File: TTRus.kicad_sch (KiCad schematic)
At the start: 90 parts, among them J1 Conn_01x05_Pin, J10 Conn_02x02_Odd_Even, J11 Conn_02x02_Odd_Even, J12 Conn_02x02_Odd_Even, J13 Conn_02x02_Odd_Even, J14 Conn_02x02_Odd_Even, J15 Conn_02x02_Odd_Even, J16 Conn_02x02_Odd_Even, J2 Conn_01x03_Pin, J3 Conn_02x02_Odd_Even, J4 Conn_02x02_Odd_Even, J5 Conn_02x02_Odd_Even, J6 Conn_02x02_Odd_Even, J7 Conn_02x02_Odd_Even, J8 Conn_02x02_Odd_Even, J9 Conn_02x02_Odd_Even, M1 Module:uaefi/0.2, P1 RT-01T-1.0B, P10 RT-01T-1.0B, P11 RT-01T-1.0B, P12 RT-01T-1.0B, P13 RT-01T-1.0B, P14 RT-01T-1.0B, P15 RT-01T-1.0B, P16 RT-01T-1.0B, P17 RT-01T-1.0B, P18 RT-01T-1.0B, P19 RT-01T-1.0B, P2 RT-01T-1.0B, P20 RT-01T-1.0B, P21 RT-01T-1.0B, P22 RT-01T-1.0B, P23 RT-01T-1.0B, P24 RT-01T-1.0B, P25 RT-01T-1.0B, P26 RT-01T-1.0B, P27 RT-01T-1.0B, P28 RT-01T-1.0B, P29 RT-01T-1.0B, P3 RT-01T-1.0B, P30 RT-01T-1.0B, P31 RT-01T-1.0B, P32 RT-01T-1.0B, P33 RT-01T-1.0B, P34 RT-01T-1.0B, P35 RT-01T-1.0B, P36 RT-01T-1.0B, P37 RT-01T-1.0B, P38 RT-01T-1.0B, P39 RT-01T-1.0B, P4 RT-01T-1.0B, P40 RT-01T-1.0B, P41 RT-01T-1.0B, P42 RT-01T-1.0B, P43 RT-01T-1.0B, P44 RT-01T-1.0B, P45 RT-01T-1.0B, P46 RT-01T-1.0B, P47 RT-01T-1.0B, P48 RT-01T-1.0B, P49 RT-01T-1.0B, P5 RT-01T-1.0B, P50 RT-01T-1.0B, P51 RT-01T-1.0B, P52 RT-01T-1.0B, P53 RT-01T-1.0B, P54 RT-01T-1.0B, P55 RT-01T-1.0B, P56 RT-01T-1.0B, P57 RT-01T-1.0B, P58 RT-01T-1.0B, P59 RT-01T-1.0B, P6 RT-01T-1.0B, P60 RT-01T-1.0B, P61 RT-01T-1.0B, P62 RT-01T-1.0B, P63 RT-01T-1.0B, P64 RT-01T-1.0B, P65 RT-01T-1.0B, P66 RT-01T-1.0B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

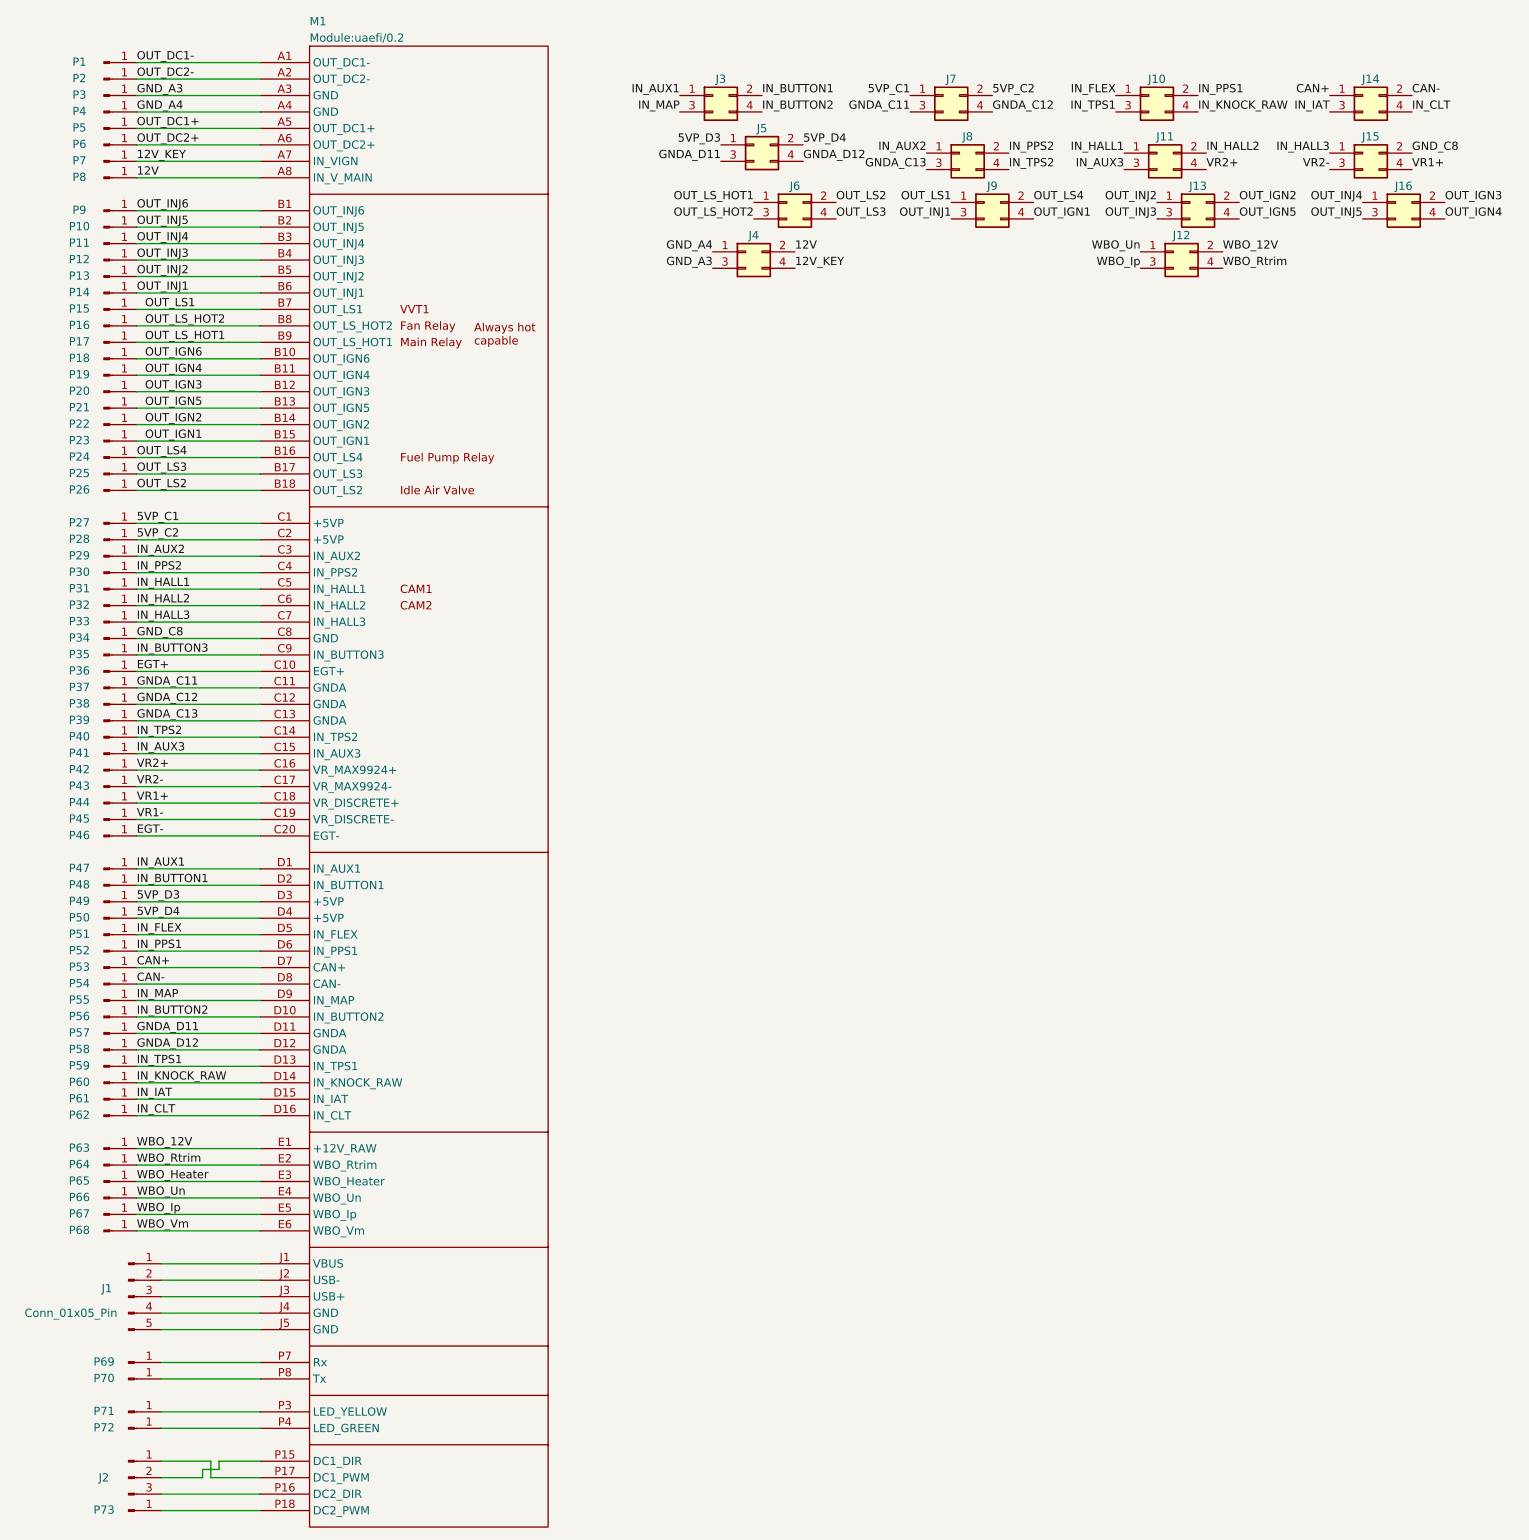
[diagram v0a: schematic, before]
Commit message: Add files via upload
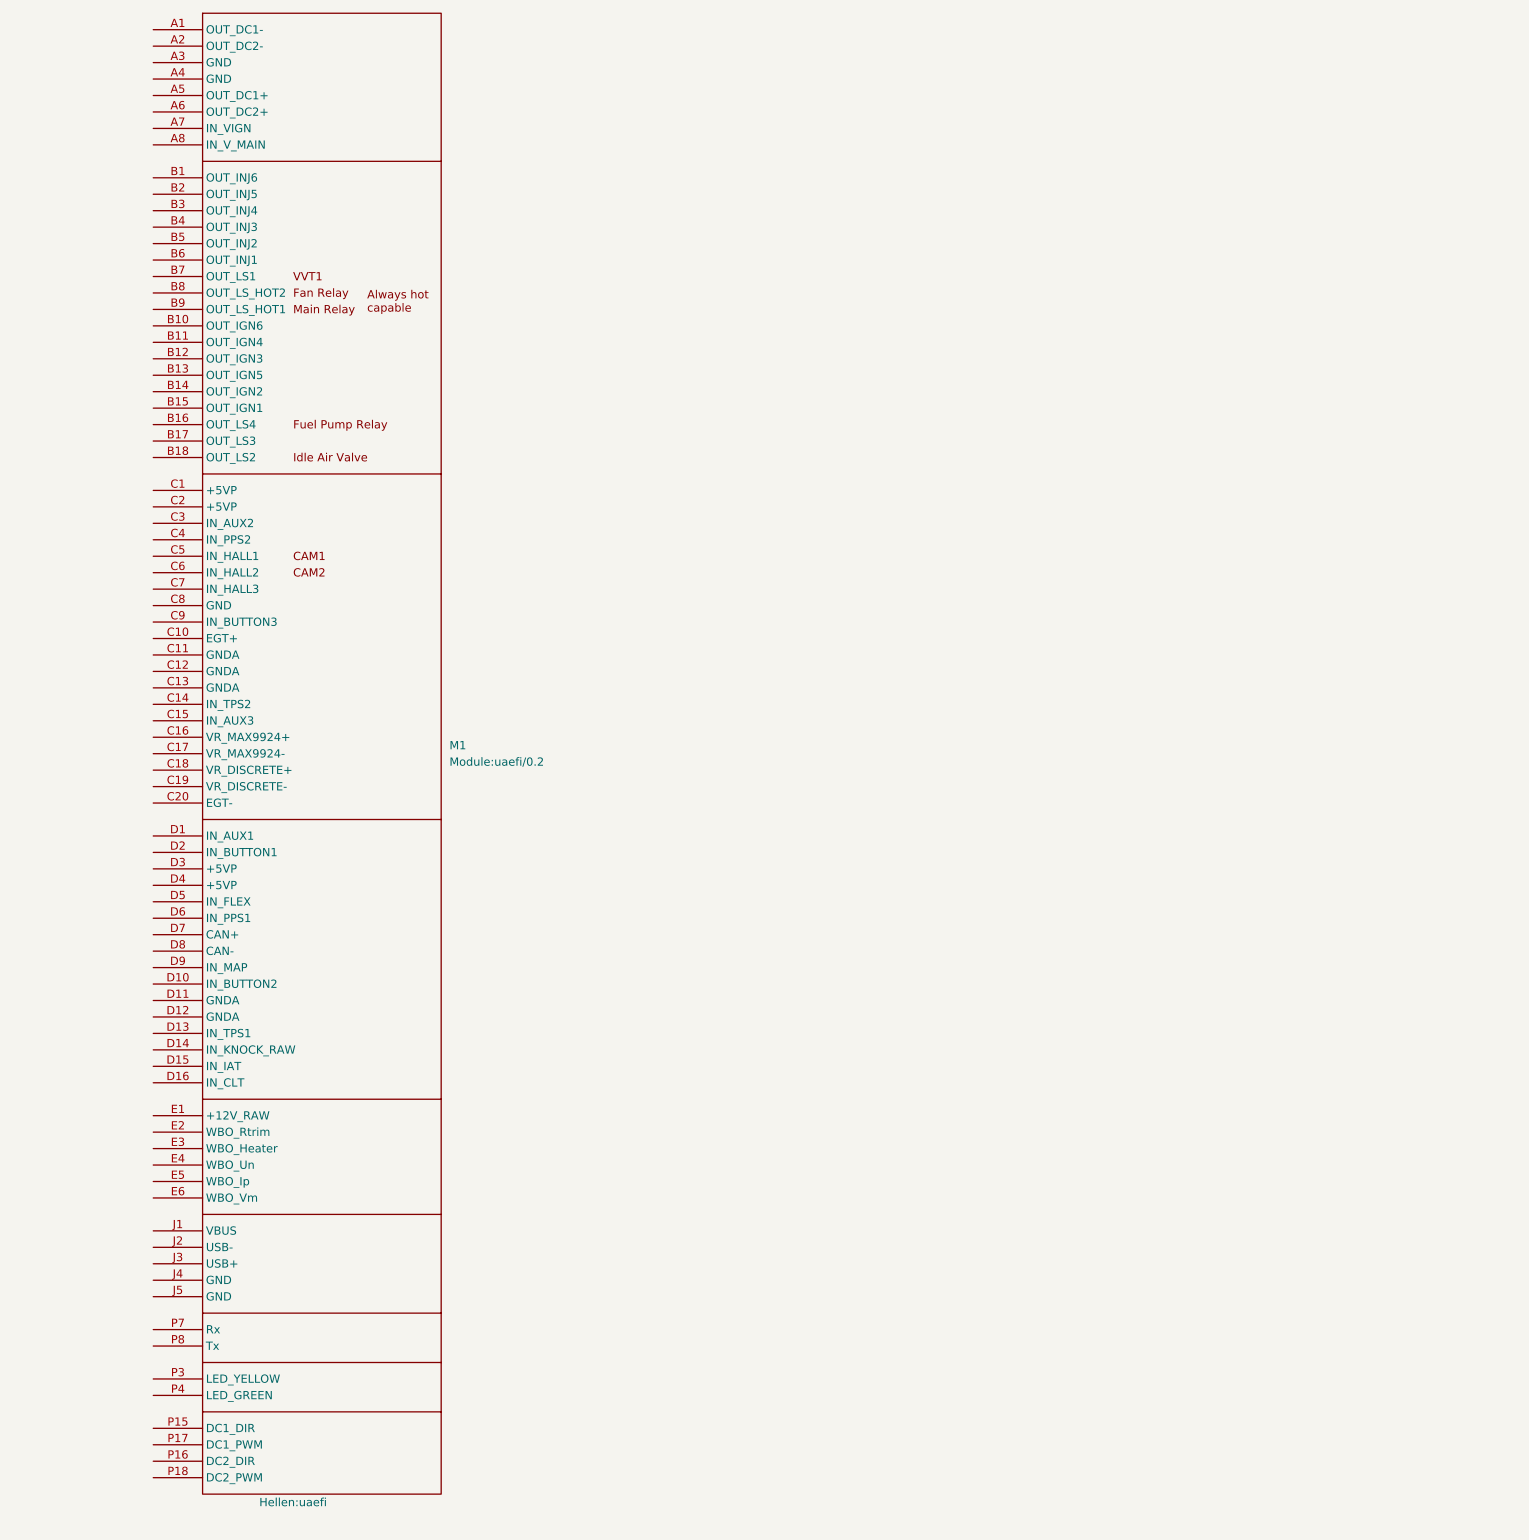
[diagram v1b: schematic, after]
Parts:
- removed J1: Conn_01x05_Pin, Connector_Molex:Molex_SPOX_5267-05A_1x05_P2.50mm_Vertical, symbol Connector:Conn_01x05_Pin
- removed J10, J11, J12, J13, J14, J15, J16, J3, J4, J5, J6, J7, J8, J9: Conn_02x02_Odd_Even, RT-01T-1.0B:2x2_2.54, symbol Connector_Generic:Conn_02x02_Odd_Even
- removed J2: Conn_01x03_Pin, RT-01T-1.0B:1x3_2.54, symbol Connector:Conn_01x03_Pin
- removed P1, P10, P11, P12, P13, P14, P15, P16, P17, P18, P19, P2, P20, P21, P22, P23, P24, P25, P26, P27, P28, P29, P3, P30, P31, P32, P33, P34, P35, P36, P37, P38, P39, P4, P40, P41, P42, P43, P44, P45, P46, P47, P48, P49, P5, P50, P51, P52, P53, P54, P55, P56, P57, P58, P59, P6, P60, P61, P62, P63, P64, P65, P66, P67, P68, P7, P8, P9: RT-01T-1.0B, RT-01T-1.0B:RT-01T-1.0B, symbol Connector:Conn_01x01_Pin
- removed P69, P70, P71, P72, P73: Conn_01x01_Pin, RT-01T-1.0B:1x1, symbol Connector:Conn_01x01_Pin
- M1: footprint hellen-one-uaefi-0.2:uaefi -> Hellen:uaefi
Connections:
- net 12V: no longer names the net of M1.A8 (IN_V_MAIN)
- net 12V_KEY: no longer names the net of M1.A7 (IN_VIGN)
- net 5VP_C1: no longer names the net of M1.C1 (+5VP)
- net 5VP_C2: no longer names the net of M1.C2 (+5VP)
- net 5VP_D3: no longer names the net of M1.D3 (+5VP)
- net 5VP_D4: no longer names the net of M1.D4 (+5VP)
- net CAN+: no longer names the net of M1.D7 (CAN+)
- net CAN-: no longer names the net of M1.D8 (CAN-)
- net EGT+: no longer names the net of M1.C10 (EGT+)
- net EGT-: no longer names the net of M1.C20 (EGT-)
- net GNDA_C11: no longer names the net of M1.C11 (GNDA)
- net GNDA_C12: no longer names the net of M1.C12 (GNDA)
- net GNDA_C13: no longer names the net of M1.C13 (GNDA)
- net GNDA_D11: no longer names the net of M1.D11 (GNDA)
- net GNDA_D12: no longer names the net of M1.D12 (GNDA)
- net GND_A3: no longer names the net of M1.A3 (GND)
- net GND_A4: no longer names the net of M1.A4 (GND)
- net GND_C8: no longer names the net of M1.C8 (GND)
- net IN_AUX1: no longer names the net of M1.D1 (IN_AUX1)
- net IN_AUX2: no longer names the net of M1.C3 (IN_AUX2)
- net IN_AUX3: no longer names the net of M1.C15 (IN_AUX3)
- net IN_BUTTON1: no longer names the net of M1.D2 (IN_BUTTON1)
- net IN_BUTTON2: no longer names the net of M1.D10 (IN_BUTTON2)
- net IN_BUTTON3: no longer names the net of M1.C9 (IN_BUTTON3)
- net IN_CLT: no longer names the net of M1.D16 (IN_CLT)
- net IN_FLEX: no longer names the net of M1.D5 (IN_FLEX)
- net IN_HALL1: no longer names the net of M1.C5 (IN_HALL1)
- net IN_HALL2: no longer names the net of M1.C6 (IN_HALL2)
- net IN_HALL3: no longer names the net of M1.C7 (IN_HALL3)
- net IN_IAT: no longer names the net of M1.D15 (IN_IAT)
- net IN_KNOCK_RAW: no longer names the net of M1.D14 (IN_KNOCK_RAW)
- net IN_MAP: no longer names the net of M1.D9 (IN_MAP)
- net IN_PPS1: no longer names the net of M1.D6 (IN_PPS1)
- net IN_PPS2: no longer names the net of M1.C4 (IN_PPS2)
- net IN_TPS1: no longer names the net of M1.D13 (IN_TPS1)
- net IN_TPS2: no longer names the net of M1.C14 (IN_TPS2)
- net OUT_DC1+: no longer names the net of M1.A5 (OUT_DC1+)
- net OUT_DC1-: no longer names the net of M1.A1 (OUT_DC1-)
- net OUT_DC2+: no longer names the net of M1.A6 (OUT_DC2+)
- net OUT_DC2-: no longer names the net of M1.A2 (OUT_DC2-)
- net OUT_IGN1: no longer names the net of M1.B15 (OUT_IGN1)
- net OUT_IGN2: no longer names the net of M1.B14 (OUT_IGN2)
- net OUT_IGN3: no longer names the net of M1.B12 (OUT_IGN3)
- net OUT_IGN4: no longer names the net of M1.B11 (OUT_IGN4)
- net OUT_IGN5: no longer names the net of M1.B13 (OUT_IGN5)
- net OUT_IGN6: no longer names the net of M1.B10 (OUT_IGN6)
- net OUT_INJ1: no longer names the net of M1.B6 (OUT_INJ1)
- net OUT_INJ2: no longer names the net of M1.B5 (OUT_INJ2)
- net OUT_INJ3: no longer names the net of M1.B4 (OUT_INJ3)
- net OUT_INJ4: no longer names the net of M1.B3 (OUT_INJ4)
- net OUT_INJ5: no longer names the net of M1.B2 (OUT_INJ5)
- net OUT_INJ6: no longer names the net of M1.B1 (OUT_INJ6)
- net OUT_LS1: no longer names the net of M1.B7 (OUT_LS1)
- net OUT_LS2: no longer names the net of M1.B18 (OUT_LS2)
- net OUT_LS3: no longer names the net of M1.B17 (OUT_LS3)
- net OUT_LS4: no longer names the net of M1.B16 (OUT_LS4)
- net OUT_LS_HOT1: no longer names the net of M1.B9 (OUT_LS_HOT1)
- net OUT_LS_HOT2: no longer names the net of M1.B8 (OUT_LS_HOT2)
- net VR1+: no longer names the net of M1.C18 (VR_DISCRETE+)
- net VR1-: no longer names the net of M1.C19 (VR_DISCRETE-)
- net VR2+: no longer names the net of M1.C16 (VR_MAX9924+)
- net VR2-: no longer names the net of M1.C17 (VR_MAX9924-)
- net WBO_12V: no longer names the net of M1.E1 (+12V_RAW)
- net WBO_Heater: no longer names the net of M1.E3 (WBO_Heater)
- net WBO_Ip: no longer names the net of M1.E5 (WBO_Ip)
- net WBO_Rtrim: no longer names the net of M1.E2 (WBO_Rtrim)
- net WBO_Un: no longer names the net of M1.E4 (WBO_Un)
- net WBO_Vm: no longer names the net of M1.E6 (WBO_Vm)
